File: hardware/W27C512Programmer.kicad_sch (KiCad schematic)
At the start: 96 parts, among them J1 CTRL, J2 MSB, J3 LSB, J4 Ext_UART, J5 OLED, J6 VP, Q1 MMBT3904, Q2 MMBT3906, Q3 MMBT3904, Q4 MMBT3904, Q5 MMBT3904, Q6 MMBT3906, Q7 MMBT3906, Q8 MMBT3906, SW1 RST, SW2 USR, U1 MIC2288, U2 74HC573, U3 74HC573, U4 74HC573, U5 28/32 pin ROM

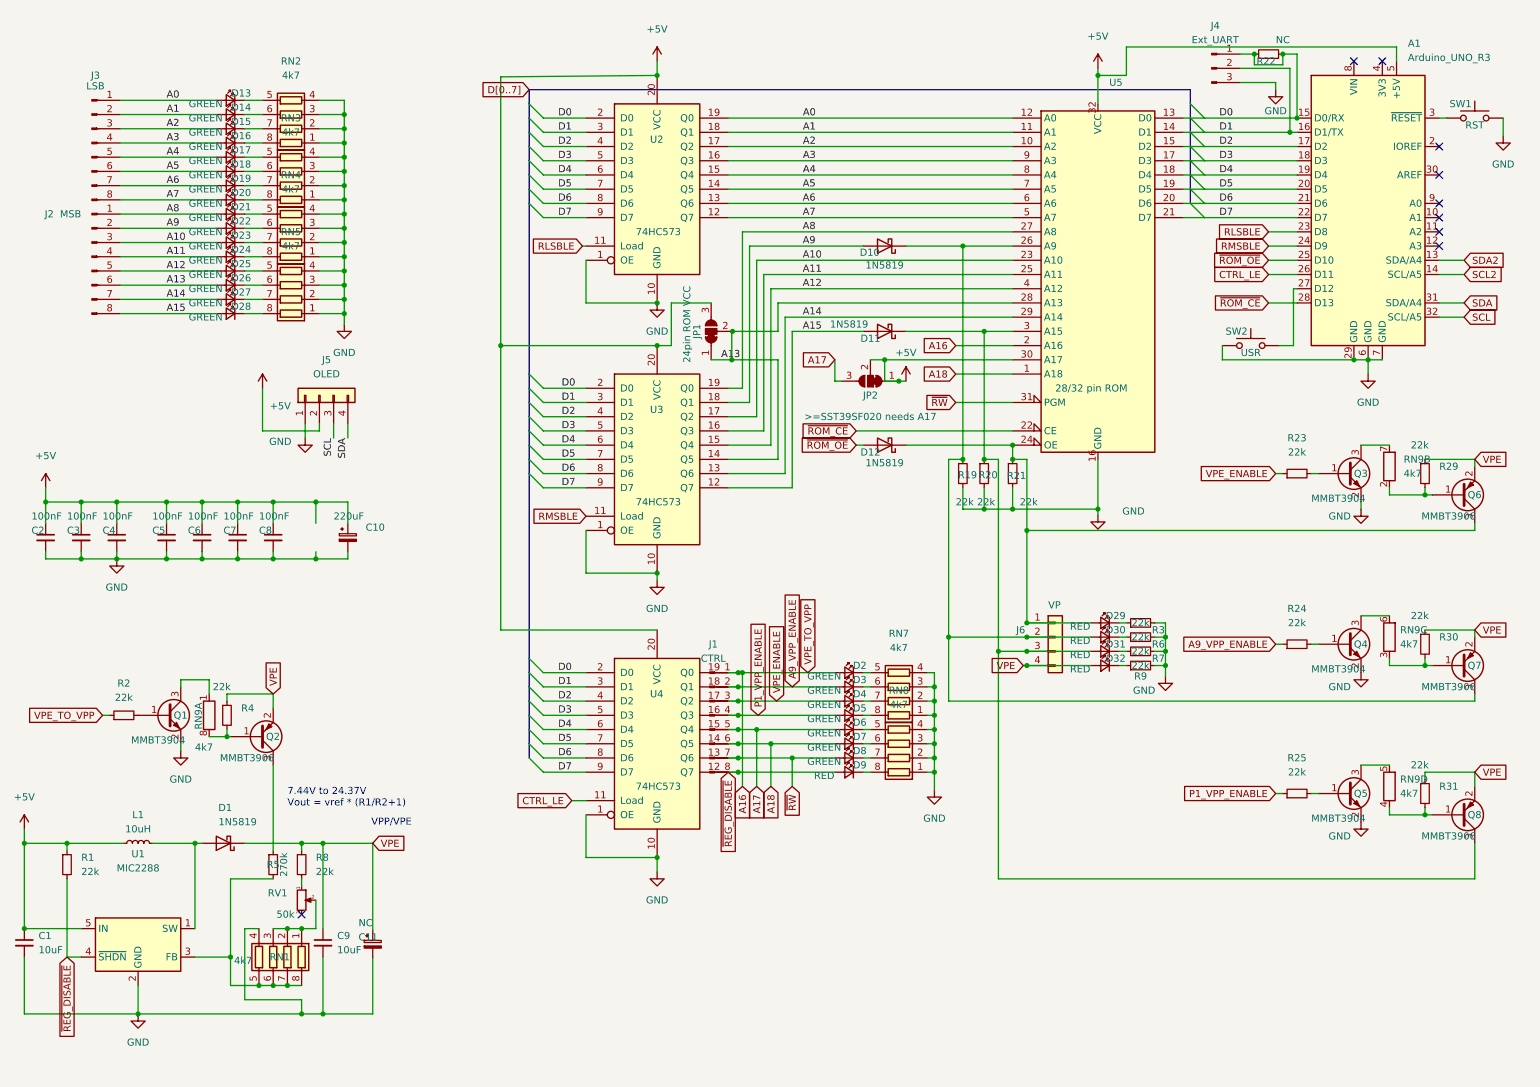
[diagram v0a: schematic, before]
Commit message: Hardware release day update!
Gerber files (zip) BOM, placement and KiCAD files as they are for Rev0
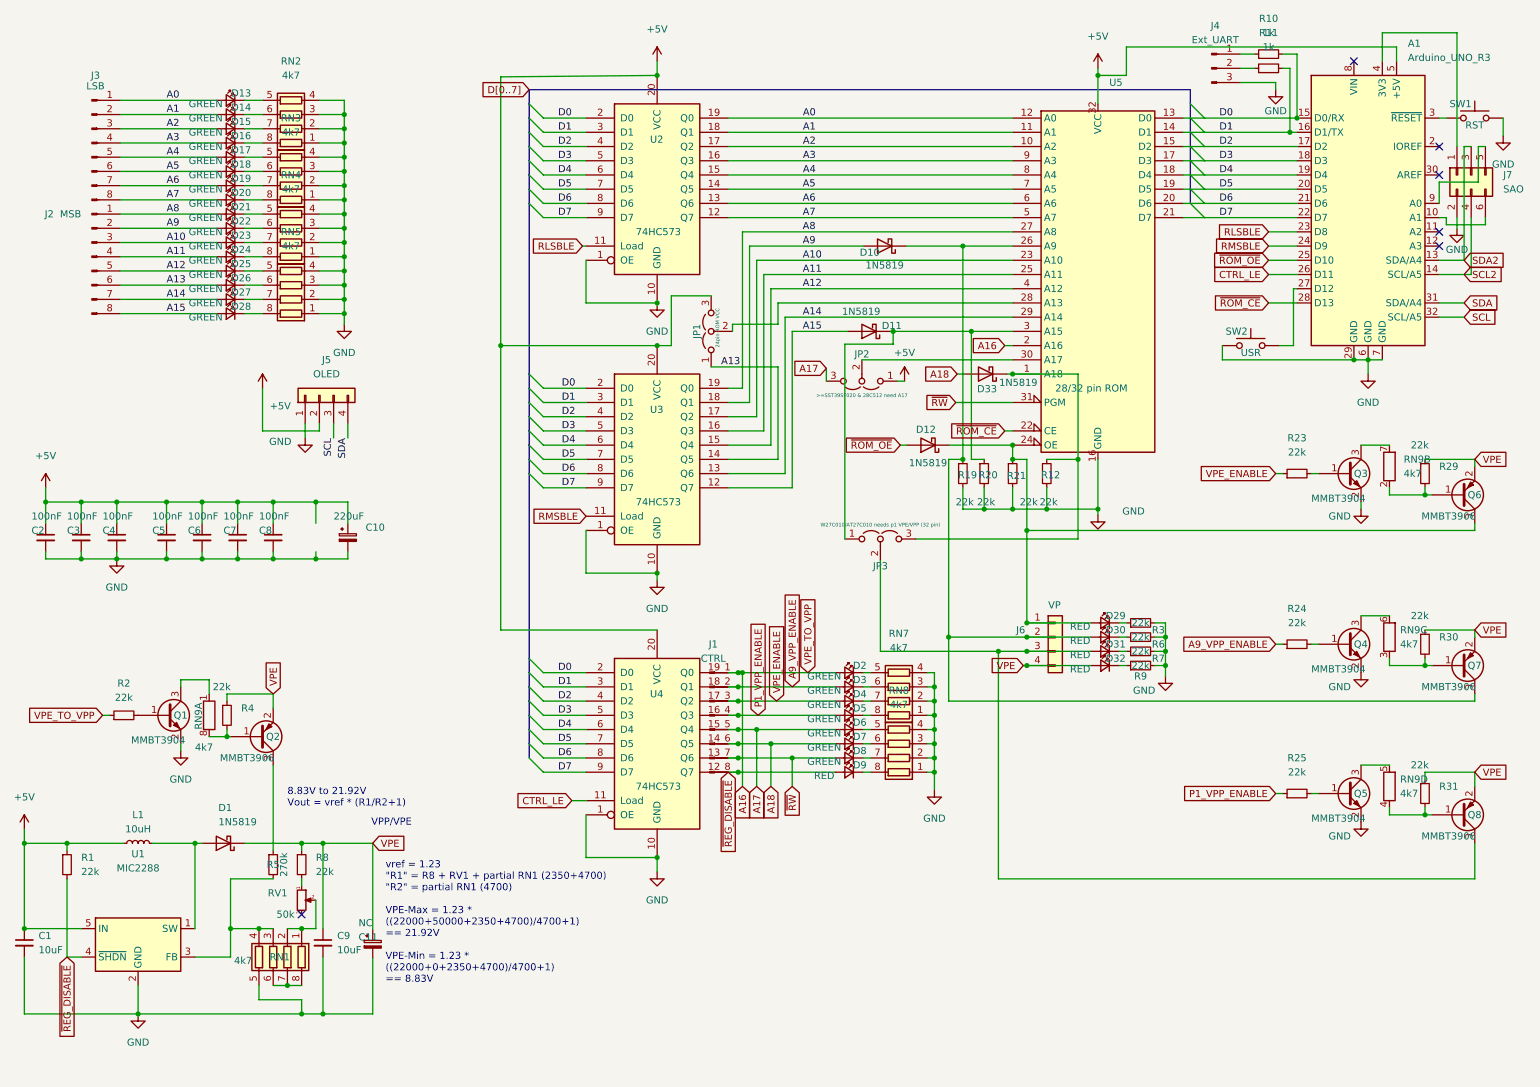
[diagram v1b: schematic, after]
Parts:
- removed R22: NC, Resistor_SMD:R_0603_1608Metric, symbol Device:R_Small
- added D33: 1N5819, Diode_SMD:D_SOD-323, symbol Diode:1N5819
- added J7: SAO, Connector_PinHeader_2.54mm:PinHeader_2x03_P2.54mm_Vertical, symbol Connector_Generic:Conn_02x03_Odd_Even
- added JP3: W27C010/AT27C010 needs p1 VPE/VPP (32 pin), Jumper:SolderJumper-3_P1.3mm_Open_RoundedPad1.0x1.5mm, symbol Jumper:Jumper_3_Open
- added R10, R11: 1k, Resistor_SMD:R_0603_1608Metric, symbol Device:R_Small
- added R12: 22k, Resistor_SMD:R_0603_1608Metric, symbol Device:R_Small
- C10: LCSC (none) -> C131120
- D13, D14, D15, D16, D17, D18, D19, D2, D20, D21, D22, D23, D24, D25, D26, D27, D28, D3, D4, D5, D6, D7, D8: LCSC (none) -> C2297
- JP1: footprint Connector_PinHeader_2.54mm:PinHeader_1x03_P2.54mm_Vertical -> Connector_PinHeader_2.54mm:PinHeader_1x03_P2.54mm_Vertical_SolderJumpers; symbol Jumper:SolderJumper_3_Bridged12 -> Jumper:Jumper_3_Open
- JP2: value >=SST39SF020 needs A17 -> >=SST39SF020 & 28C512 need A17; footprint Connector_PinHeader_2.54mm:PinHeader_1x03_P2.54mm_Vertical -> Connector_PinHeader_2.54mm:PinHeader_1x03_P2.54mm_Vertical_SolderJumpers; symbol Jumper:SolderJumper_3_Bridged12 -> Jumper:Jumper_3_Open
- Q1, Q3, Q4, Q5: LCSC (none) -> C20526
- Q2, Q6, Q7, Q8: LCSC (none) -> C7420354
- RN1, RN2, RN3, RN4, RN5, RN7, RN8, RN9: LCSC (none) -> C1980
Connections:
- net +5V: no longer JP2.2 (C), U5.30 (A17)
- net A13: no longer JP1.2 (C), U5.28 (A13)
- net A18: now also D33.2 (A); no longer U5.1 (A18)
- net D0: now also R10.2; no longer J4.1 (Pin_1)
- net D1: now also R11.2; no longer J4.2 (Pin_2)
- net GND: now also RN1.5 (R4.2), J7.2 (Pin_2), R12.2; no longer RN1.4 (R4.1)
- net SCL2: now also J7.4 (Pin_4)
- net SDA2: now also J7.3 (Pin_3)
- net at D11.1 (K), R20.1, U5.3 (A15): now also JP3.1 (A); no longer D31.2 (A), J6.3 (Pin_3), Q8.3 (C)
- net at RN1.6 (R3.2), RN1.7 (R2.2), RN1.8 (R1.2): no longer R5.2, RN1.5 (R4.2), U1.3 (FB)
- net at RN1.1 (R1.1), RN1.2 (R2.1), RV1.2: no longer RN1.3 (R3.1)
- net at A1.10 (A1): now also J7.6 (Pin_6)
- net at A1.4 (3V3): now also J7.1 (Pin_1)
- net at A1.9 (A0): now also J7.5 (Pin_5)
- new net: D31.2 (A), J6.3 (Pin_3), JP3.2 (C), Q8.3 (C)
- new net: J4.2 (Pin_2), R11.1
- new net: R5.2, RN1.3 (R3.1), RN1.4 (R4.1), U1.3 (FB)
- new net: J4.1 (Pin_1), R10.1
- new net: D33.1 (K), JP3.3 (B), R12.1, U5.1 (A18)
- new net: JP1.2 (C), U5.28 (A13)
- new net: JP2.2 (C), U5.30 (A17)
- no-connect marks 9 -> 6
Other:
- note added: "8.83V to 21.92V Vout = vref * (R1/R2+1)"
- note added: "vref = 1.23 "R1" = R8 + RV1 + partial RN1 (2350+4700) "R2" = partial RN1 (4700) VPE-Max = 1.23 * ((22000+50000+2350+4700)/4700+1) == 21.92V VPE-Min = 1.23 * ((22000+0+2350+4700)/4700+1) == 8.83V"
- note removed: "7.44V to 24.37V Vout = vref * (R1/R2+1)"
- moved on the sheet: D11, D12
